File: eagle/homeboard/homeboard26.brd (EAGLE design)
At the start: 94 x 71.8 mm, 124 parts, among them IC1 XCF02S, IC2 25LC080SN, IC3 ATMEGA32U2-TQFP, Q5 BC848SMD, Q6 BC848SMD, Q7 BC848SMD, Q8 BC848SMD, T1 BSS138, T2 BC848, T3 BSS138, U1 XC3S400TQ144, X1 SCART-CLIP, X6 MINI-USB_4P-85-32004-10X, X7 DC21MMX, X8 STEREOJACK

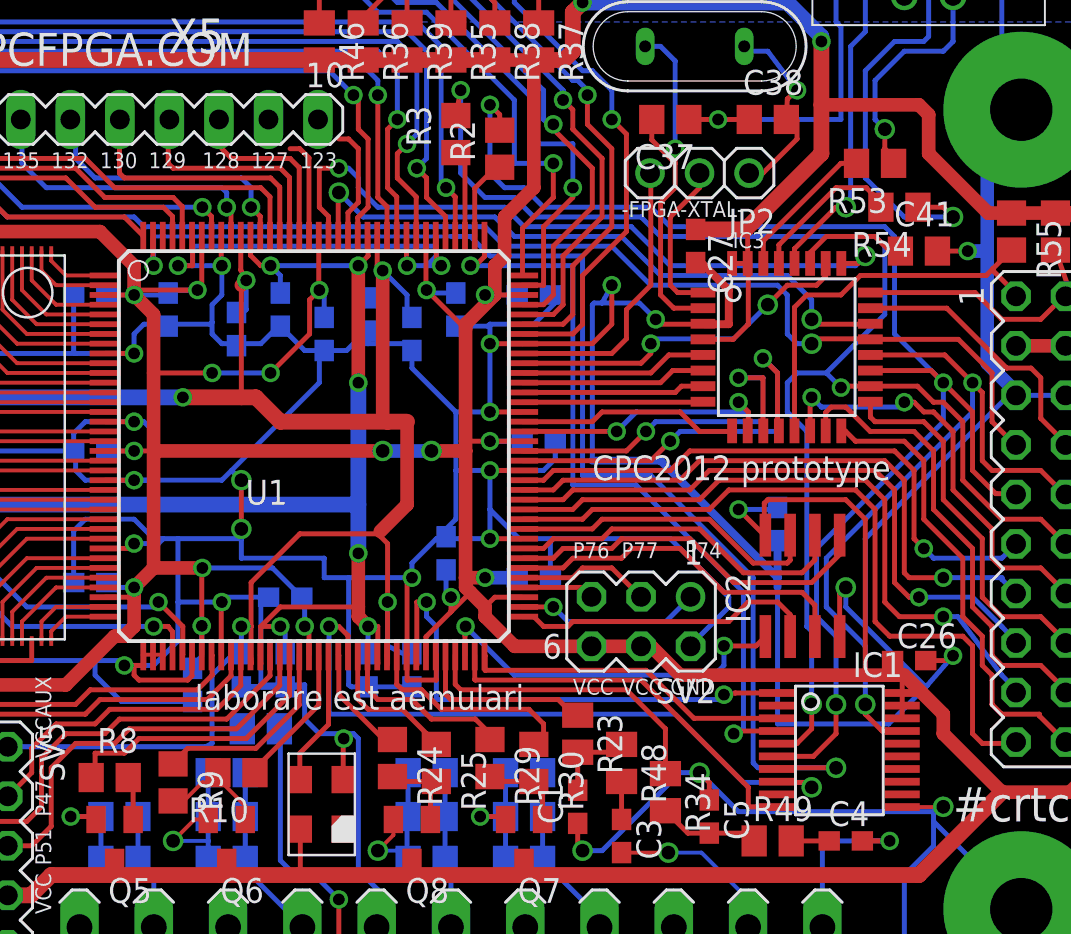
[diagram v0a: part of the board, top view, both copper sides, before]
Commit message: about to add ground planes
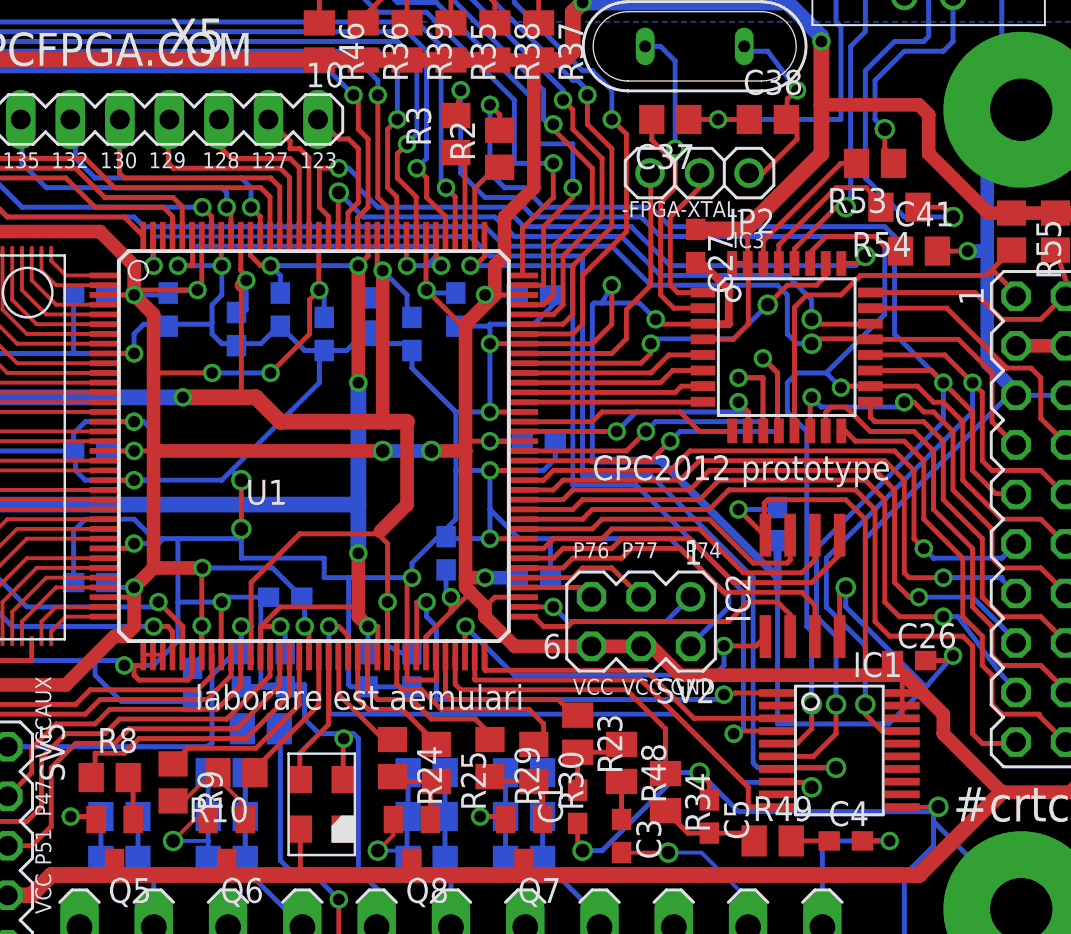
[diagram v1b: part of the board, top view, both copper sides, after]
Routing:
- net N$7: track 5.24 -> 7.20 mm
- net N$6: track 7.95 -> 9.51 mm
- net N$16: track 5.98 -> 7.39 mm
- net N$5: track 11.3 -> 11.9 mm
- net N$4: track 13.3 -> 13.9 mm
- net GND: track 992.5 -> 992.0 mm
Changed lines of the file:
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@@
 <wire x1="68" y1="13" x2="72" y2="17" width="0.254" layer="16"/>
 <wire x1="72" y1="17" x2="73" y2="17" width="0.254" layer="16"/>
-<wire x1="83.393396875" y1="15.237409375" x2="85.487409375" y2="15.237409375" width="0.2" layer="1"/>
-<wire x1="85.487409375" y1="15.237409375" x2="85.5" y2="15.25" width="0.2" layer="1"/>
-<via x="85.5" y="15.25" extent="1-16" drill="0.7" shape="square"/>
-<wire x1="85.5" y1="15.25" x2="85.25" y2="15.25" width="0.2" layer="16"/>
+<wire x1="83.393396875" y1="15.237409375" x2="85.237409375" y2="15.237409375" width="0.2" layer="1"/>
+<wire x1="85.237409375" y1="15.237409375" x2="85.25" y2="15.25" width="0.2" layer="1"/>
+<via x="85.25" y="15.25" extent="1-16" drill="0.7" shape="square"/>
 <wire x1="85.25" y1="15.25" x2="85" y2="15" width="0.2" layer="16"/>
 <wire x1="89.5" y1="10" x2="85" y2="14.5" width="0.254" layer="16"/>
@@
 <wire x1="51" y1="47.5" x2="43.5" y2="47.5" width="0.254" layer="1"/>
 <wire x1="43.5" y1="47.5" x2="43.25" y2="47.75" width="0.254" layer="1"/>
-<wire x1="43.25" y1="47.75" x2="43.25" y2="49.98" width="0.254" layer="1"/>
-<wire x1="43.25" y1="49.98" x2="43.27" y2="50.5" width="0" layer="19" extent="1-16"/>
+<wire x1="43.25" y1="47.75" x2="43.25" y2="50.48" width="0.254" layer="1"/>
+<wire x1="43.25" y1="50.48" x2="43.27" y2="50.5" width="0.254" layer="1"/>
 </signal>
 <signal name="N$5">
@@
 <wire x1="51.5" y1="48" x2="46" y2="48" width="0.254" layer="1"/>
 <wire x1="46" y1="48" x2="45.75" y2="48.25" width="0.254" layer="1"/>
-<wire x1="45.75" y1="48.25" x2="45.75" y2="49.94" width="0.254" layer="1"/>
-<wire x1="45.75" y1="49.94" x2="45.81" y2="50.5" width="0" layer="19" extent="1-16"/>
+<wire x1="45.75" y1="48.25" x2="45.75" y2="50.44" width="0.254" layer="1"/>
+<wire x1="45.75" y1="50.44" x2="45.81" y2="50.5" width="0.254" layer="1"/>
 </signal>
 <signal name="N$6">
@@
 <wire x1="52" y1="48.5" x2="49" y2="48.5" width="0.254" layer="1"/>
 <wire x1="49" y1="48.5" x2="48.5" y2="49" width="0.254" layer="1"/>
-<wire x1="48.5" y1="49" x2="48.5" y2="50.5" width="0" layer="19" extent="1-16"/>
-<wire x1="48.35" y1="50.5" x2="48.5" y2="50.5" width="0" layer="19" extent="1-16"/>
+<wire x1="48.5" y1="49" x2="48.5" y2="50.35" width="0.254" layer="1"/>
+<wire x1="48.5" y1="50.35" x2="48.35" y2="50.5" width="0.254" layer="1"/>
 </signal>
 <signal name="N$7">
@@
 <wire x1="52.97" y1="48.53" x2="52.5" y2="49" width="0.254" layer="1"/>
 <wire x1="52.5" y1="49" x2="52" y2="49" width="0.254" layer="1"/>
-<wire x1="52" y1="49" x2="50.5" y2="50.5" width="0" layer="19" extent="1-16"/>
-<wire x1="50.5" y1="50.5" x2="50.89" y2="50.5" width="0" layer="19" extent="1-16"/>
-<wire x1="51" y1="50.5" x2="50.89" y2="50.5" width="0" layer="19" extent="1-16"/>
+<wire x1="52" y1="49" x2="52" y2="49.39" width="0.254" layer="1"/>
+<wire x1="52" y1="49.39" x2="50.89" y2="50.5" width="0.254" layer="1"/>
 </signal>
 <signal name="N$16">
@@
 <wire x1="55.5" y1="49" x2="55" y2="49.5" width="0.254" layer="1"/>
 <wire x1="55" y1="49.5" x2="54.5" y2="49.5" width="0.254" layer="1"/>
-<wire x1="54.5" y1="49.5" x2="53.5" y2="50.5" width="0" layer="19" extent="1-16"/>
-<wire x1="53.5" y1="50.5" x2="53.43" y2="50.5" width="0" layer="19" extent="1-16"/>
+<wire x1="54.5" y1="49.5" x2="53.5" y2="50.5" width="0.254" layer="1"/>
+<wire x1="53.5" y1="50.5" x2="53.43" y2="50.5" width="0" layer="19" extent="1-1"/>
 </signal>
 <signal name="N$8">
